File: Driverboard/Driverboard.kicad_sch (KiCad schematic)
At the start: 0 parts

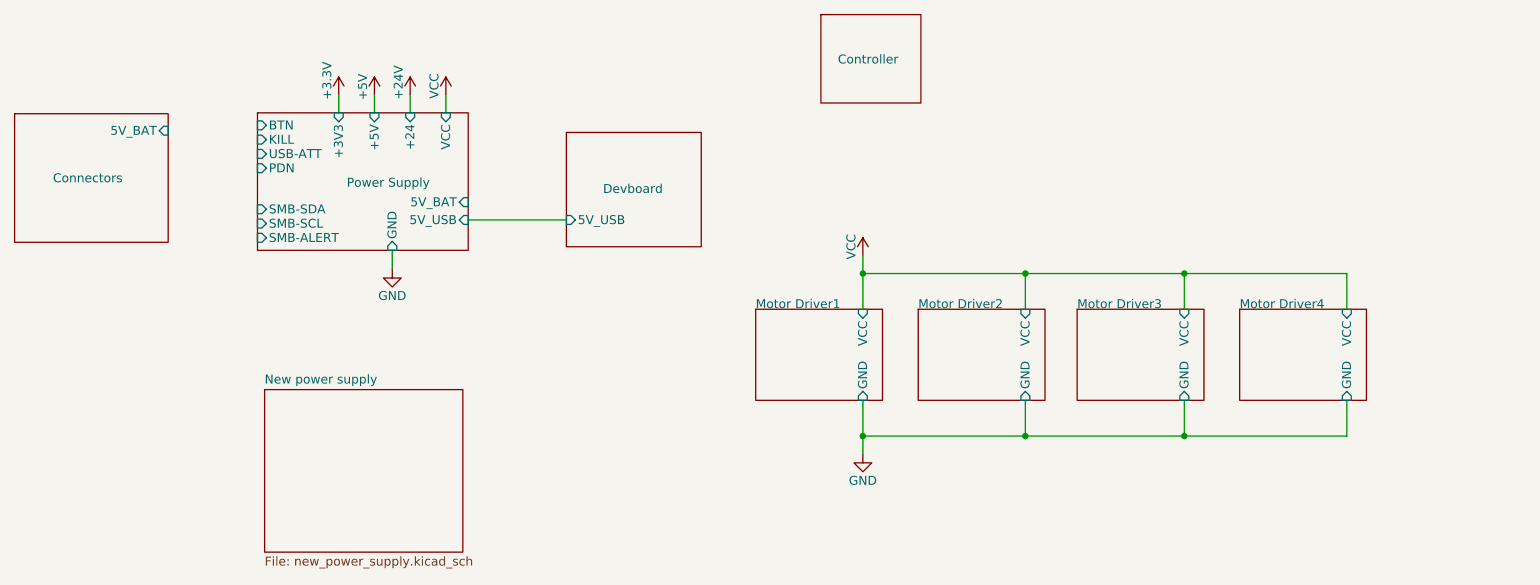
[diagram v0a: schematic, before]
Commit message: WIP
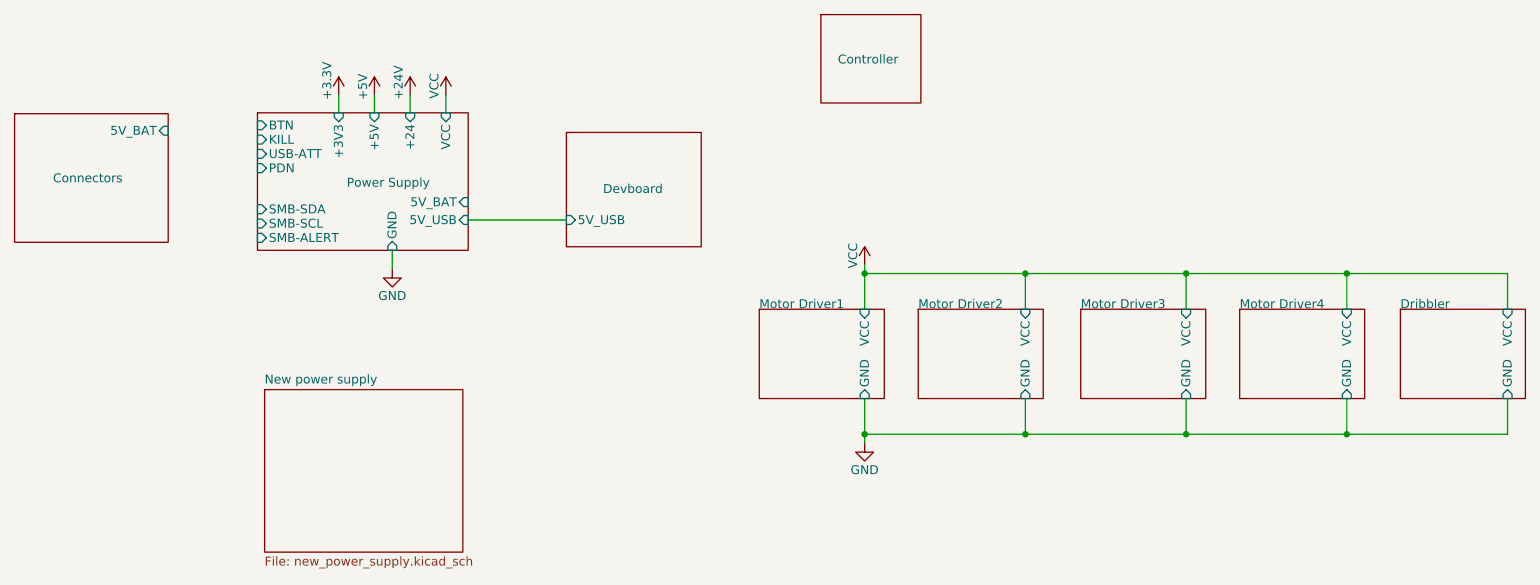
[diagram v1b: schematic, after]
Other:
- added sheet Dribbler (motor_driver.kicad_sch)
